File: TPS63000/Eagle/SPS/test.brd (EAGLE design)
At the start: 100 x 80 mm, 22 parts, among them IC1 ATXMEGA32AA, J1 USB-MICROB", J2 USB-MICROB"

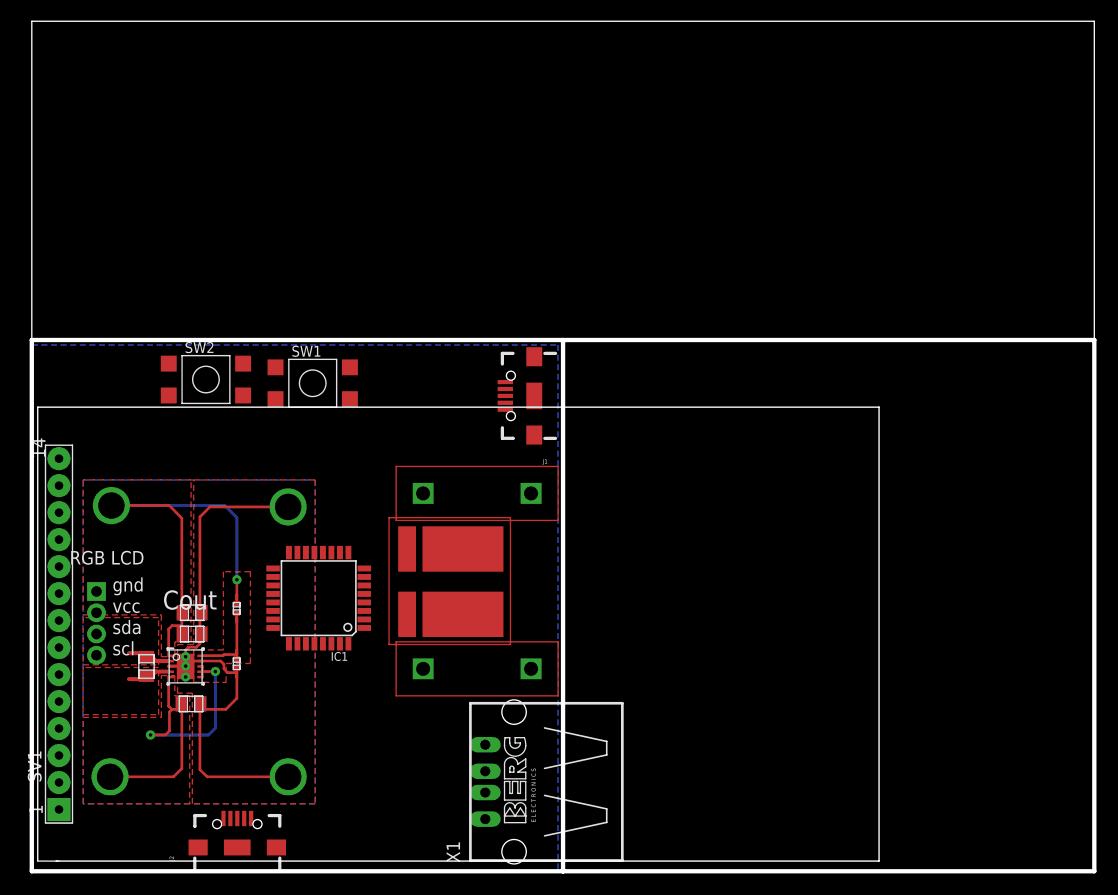
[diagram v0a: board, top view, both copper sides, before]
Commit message: updated designs
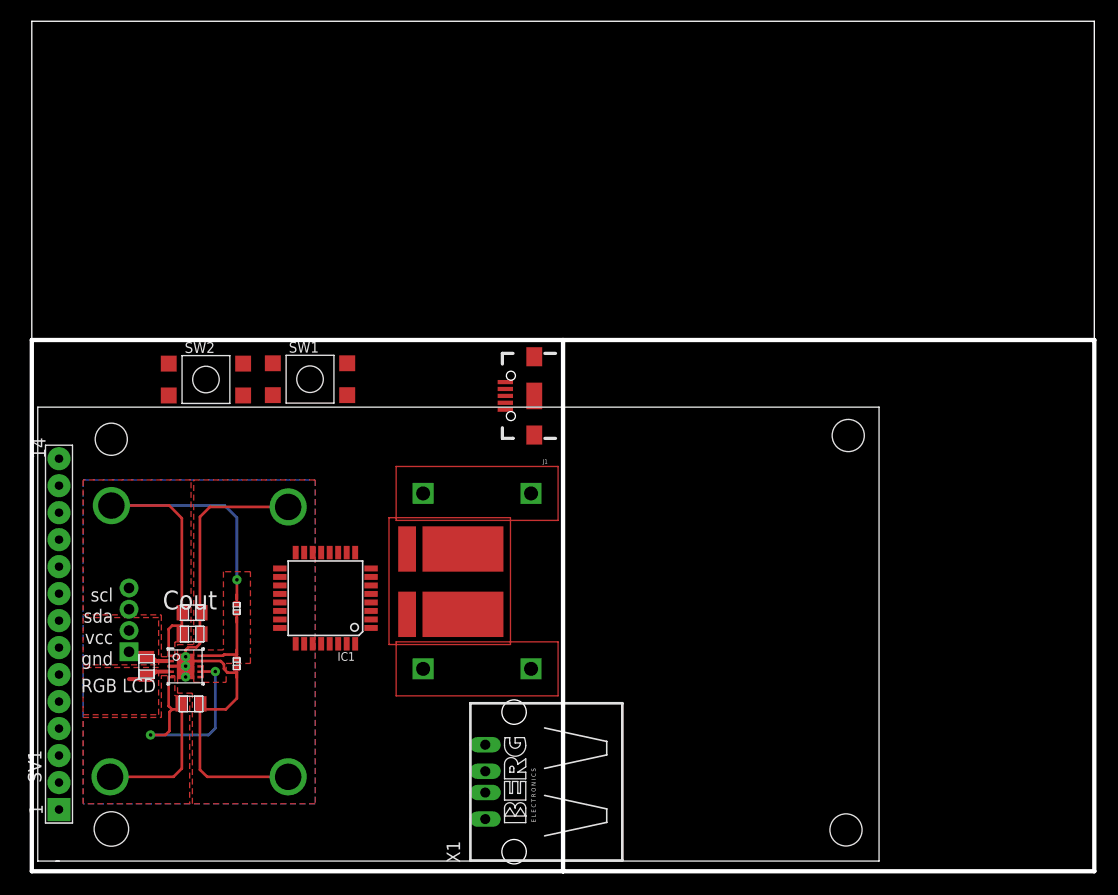
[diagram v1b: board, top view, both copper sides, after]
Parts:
- removed J2: USB-MICROB", SparkFun-Connectors:USB-B-MICRO-SMD_V03
- moved U$1 6.44 mm to (9.15, 20.7), turned to 180 degrees
- moved IC1 0.64 mm to (27.6, 25.7)
- moved SW1 0.46 mm to (26.2, 46.3)
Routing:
- removed copper zone on layer 16, net S$1
